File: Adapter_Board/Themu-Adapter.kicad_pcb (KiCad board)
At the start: 2 copper layers, 20.8 x 50.5 mm, 7 parts, among them J1 Conn_01x08, J2 LilyConn_01x02, J3 LilyConn_01x02, J4 LilyConn_01x02, J5 LilyConn_01x02, J6 LilyConn_01x02, J7 LilyConn_01x02

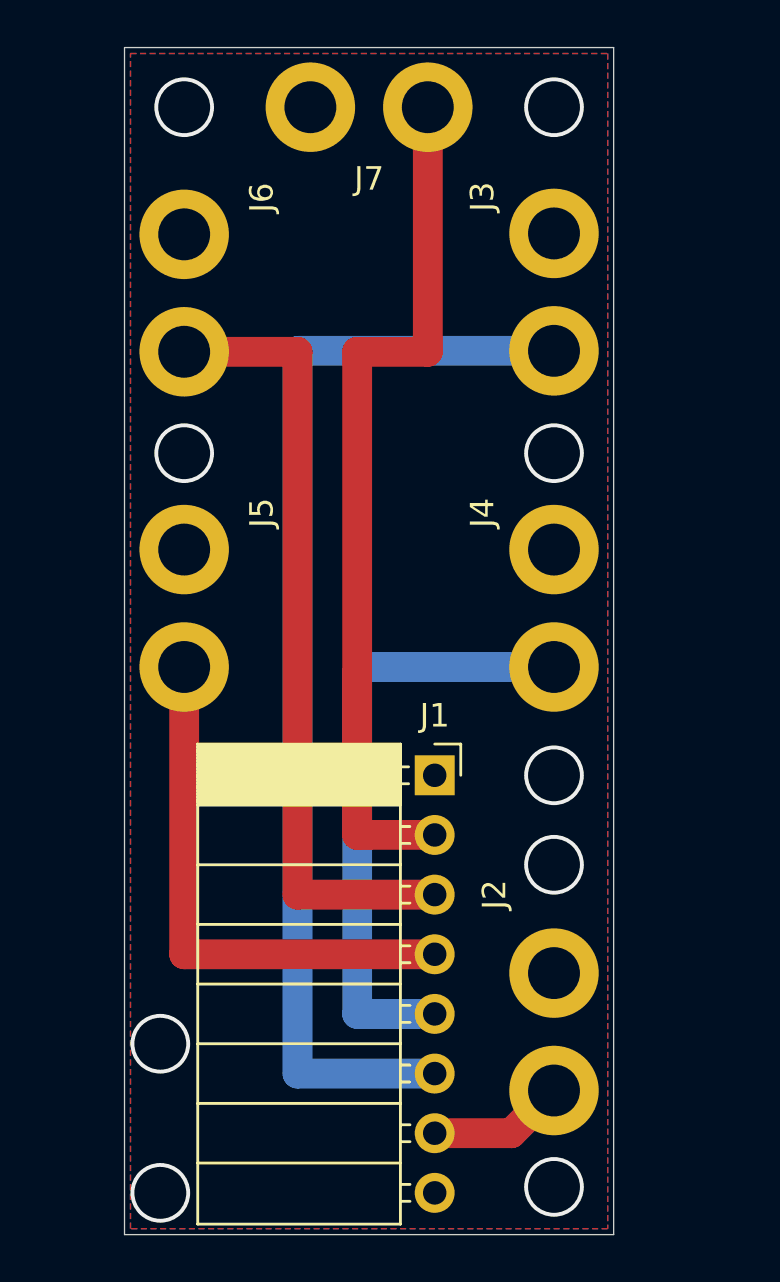
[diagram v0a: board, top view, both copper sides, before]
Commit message: Rev 2.0 commit. INTI revision.
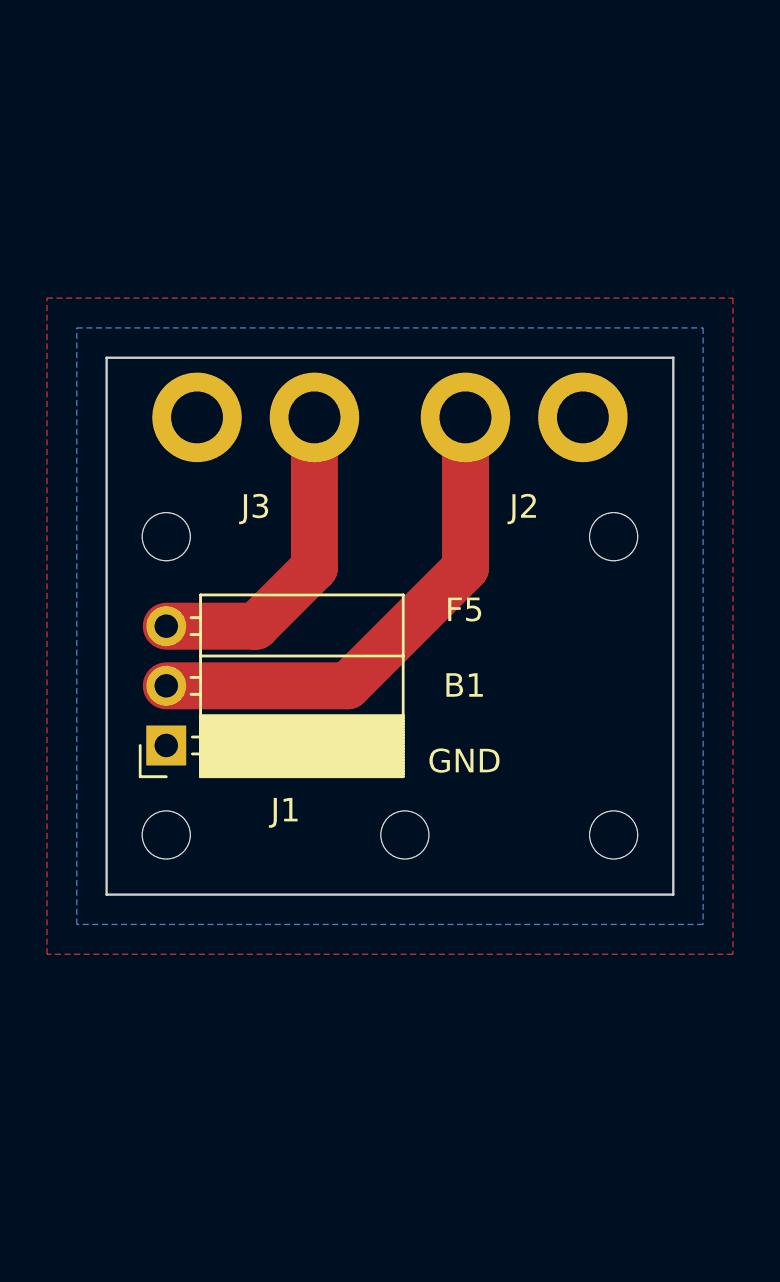
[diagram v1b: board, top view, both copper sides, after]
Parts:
- removed J4, J5, J6, J7: LilyConn_01x02, Themu-Adapter:LilyConn_01x02_87mils_130mils
- J1: value Conn_01x08 -> Conn_01x03; footprint Connector_PinSocket_2.54mm:PinSocket_1x08_P2.54mm_Horizontal -> Connector_PinSocket_2.54mm:PinSocket_1x03_P2.54mm_Horizontal
- moved J2 26.2 mm to (125.7, 50.8), turned to 180 degrees
- moved J3 13.8 mm to (114.3, 50.8), turned to 0 degrees
- moved J1 11.5 mm to (110.5, 64.8), turned to 180 degrees
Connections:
- J1 pad 1: (no net) -> GND
- J2 pad 2: /FLEX1 -> /BUTTON
- J3 pad 2: /FLEX2 -> /FLEX5
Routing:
- net /FLEX2: track 47.5 -> 0.00 mm
- net /FLEX3: track 26.3 -> 0.00 mm
- net /FLEX4: track 22.9 -> 0.00 mm
- net /FLEX5: track 33.8 -> 13.7 mm
- net /BUTTON: track 37.3 -> 21.2 mm
- net /FLEX1: track 5.83 -> 0.00 mm
- net (no net): vias 9 -> 5
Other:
- board size 20.8 x 50.5 mm -> 24.1 x 22.9 mm
- net class Default: clearance 0.2 -> 0.5; trace_width 0.25 -> 2
- rule trace_clearance: 0.2 -> 0.5
- board text added: "*Board Size: 950x900 mils (24.13x22.86 mm)"
- board text added: "F5 B1 GND"
